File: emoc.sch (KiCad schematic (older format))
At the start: 0 parts

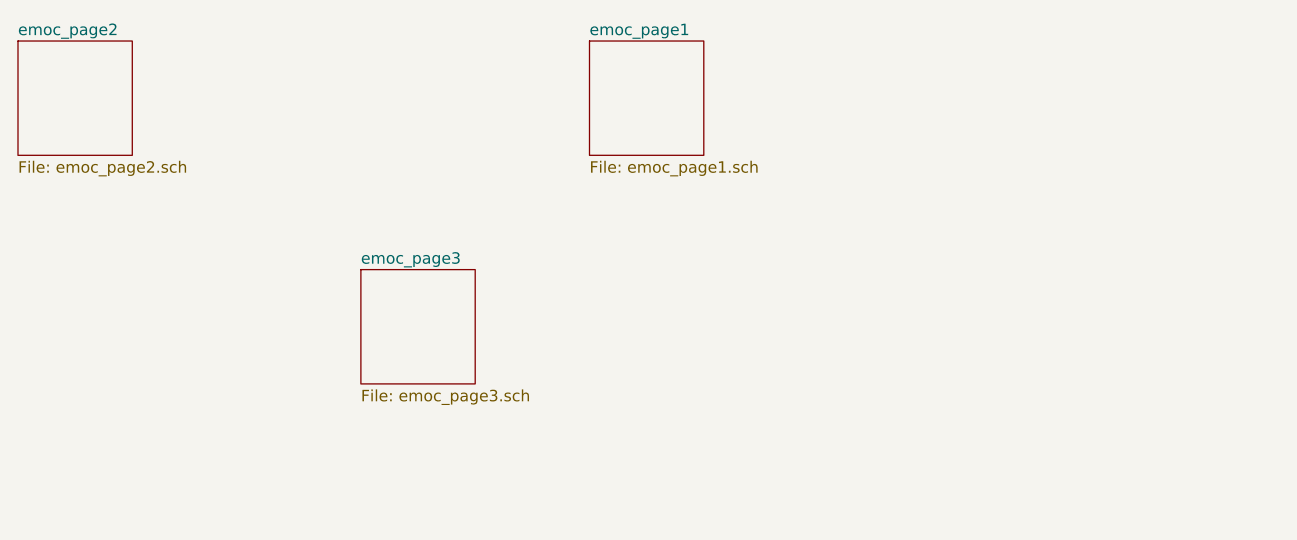
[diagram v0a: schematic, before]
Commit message: still work in progress
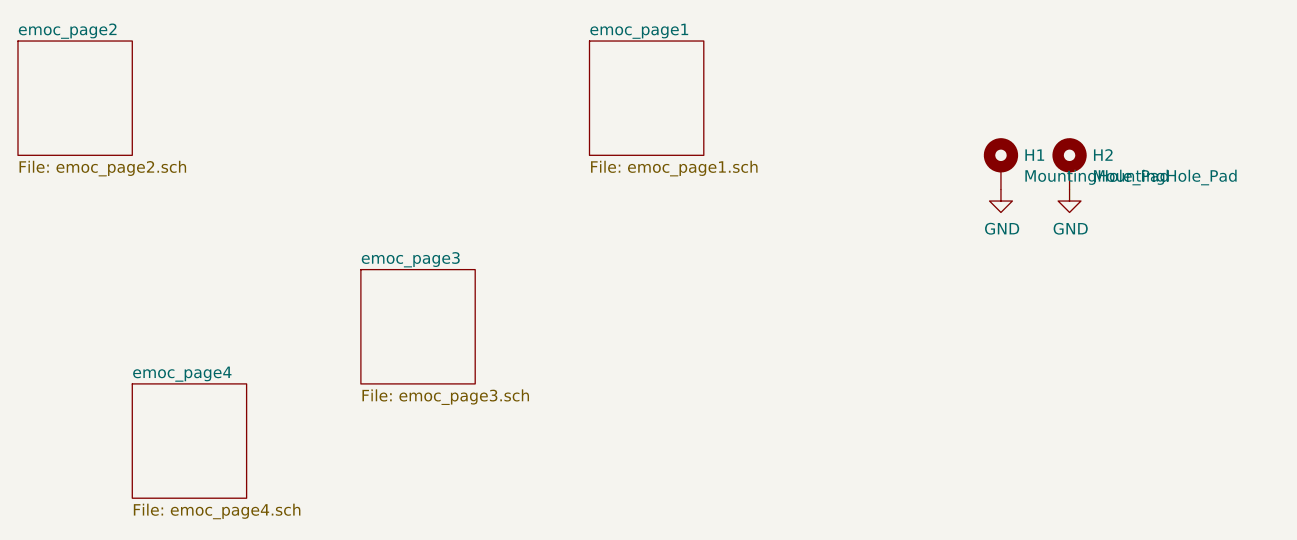
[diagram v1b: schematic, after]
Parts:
- added H1, H2: MountingHole_Pad, MountingHole:MountingHole_3.2mm_M3_Pad, symbol Mechanical:MountingHole_Pad
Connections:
- new net GND: H1.1, H2.1
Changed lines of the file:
@@
 $Descr A4 11693 8268
 encoding utf-8
-Sheet 1 4
+Sheet 1 5
 Title ""
 Date ""
@@
 F1 "emoc_page3.sch" 50
 $EndSheet
+$Sheet
+S 3000 5000 500  500
+U 5FFE6807
+F0 "emoc_page4" 50
+F1 "emoc_page4.sch" 50
+$EndSheet
+$Comp
+L Mechanical:MountingHole_Pad H1
+U 1 1 6019B66E
+P 6800 4050
+F 0 "H1" H 6900 4099 50  0000 L CNN
+F 1 "MountingHole_Pad" H 6900 4008 50  0000 L CNN
+F 2 "MountingHole:MountingHole_3.2mm_M3_Pad" H 6800 4050 50  0001 C CNN
+F 3 "~" H 6800 4050 50  0001 C CNN
+	1    6800 4050
+	1    0    0    -1
+$EndComp
+$Comp
+L power:GND #PWR0110
+U 1 1 6019BCA5
+P 6800 4150
+F 0 "#PWR0110" H 6800 3900 50  0001 C CNN
+F 1 "GND" H 6805 3977 50  0000 C CNN
+F 2 "" H 6800 4150 50  0001 C CNN
+F 3 "" H 6800 4150 50  0001 C CNN
+	1    6800 4150
+	1    0    0    -1
+$EndComp
+$Comp
+L power:GND #PWR0121
+U 1 1 6019C146
+P 7100 4150
+F 0 "#PWR0121" H 7100 3900 50  0001 C CNN
+F 1 "GND" H 7105 3977 50  0000 C CNN
+F 2 "" H 7100 4150 50  0001 C CNN
+F 3 "" H 7100 4150 50  0001 C CNN
+	1    7100 4150
+	1    0    0    -1
+$EndComp
+$Comp
+L Mechanical:MountingHole_Pad H2
+U 1 1 6032109F
+P 7100 4050
+F 0 "H2" H 7200 4099 50  0000 L CNN
+F 1 "MountingHole_Pad" H 7200 4008 50  0000 L CNN
+F 2 "MountingHole:MountingHole_3.2mm_M3_Pad" H 7100 4050 50  0001 C CNN
+F 3 "~" H 7100 4050 50  0001 C CNN
+	1    7100 4050
+	1    0    0    -1
+$EndComp
 $EndSCHEMATC
